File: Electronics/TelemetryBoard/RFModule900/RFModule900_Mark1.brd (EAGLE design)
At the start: 100 x 30 mm, 166 parts, among them T1 DC08-73, T2 DC08-73, U1 TPS2561, U2 TPS2561, U3 LM75B, U4 LTC5505, U5 LTC5505, U6 MCP4728, U7 ADC128D818, U8 MIC5504-3.3YM5, U9 TCA9535, Y1 30 Mhz

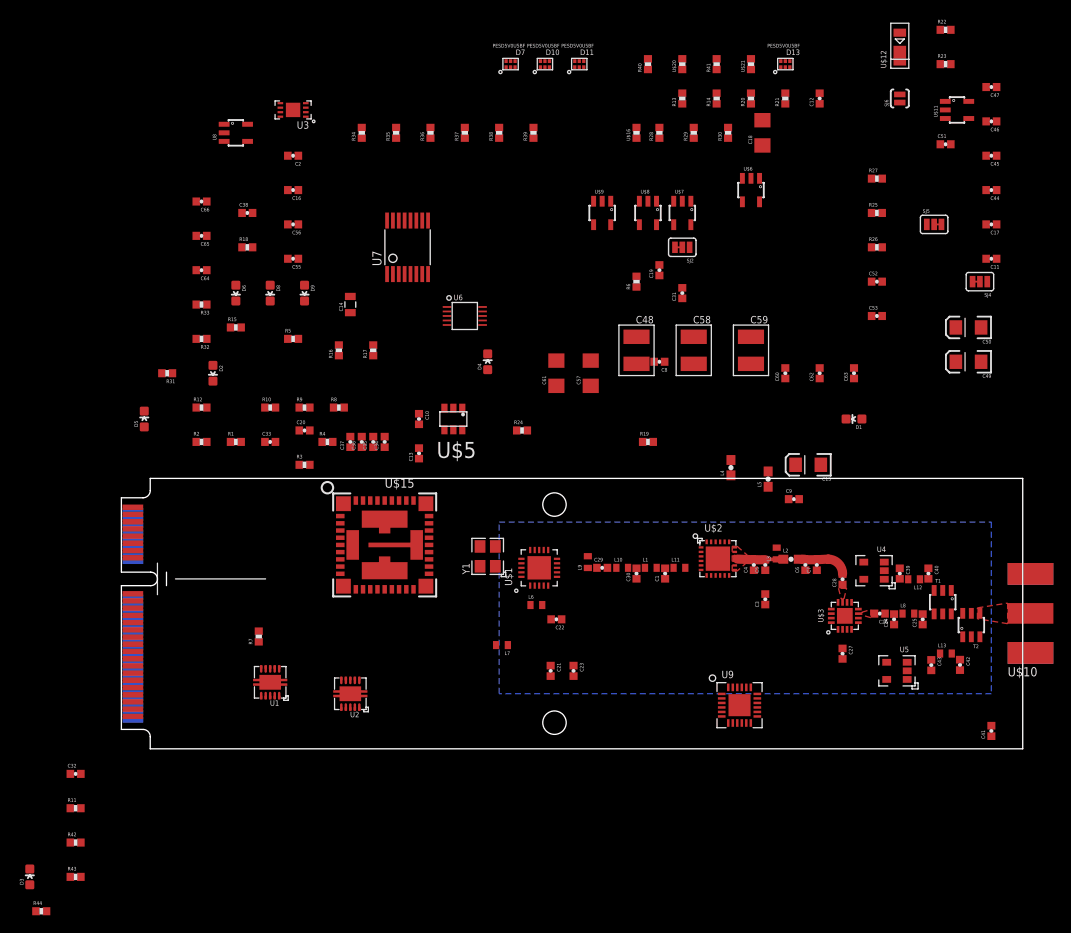
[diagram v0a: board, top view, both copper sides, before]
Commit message: Working on routing board
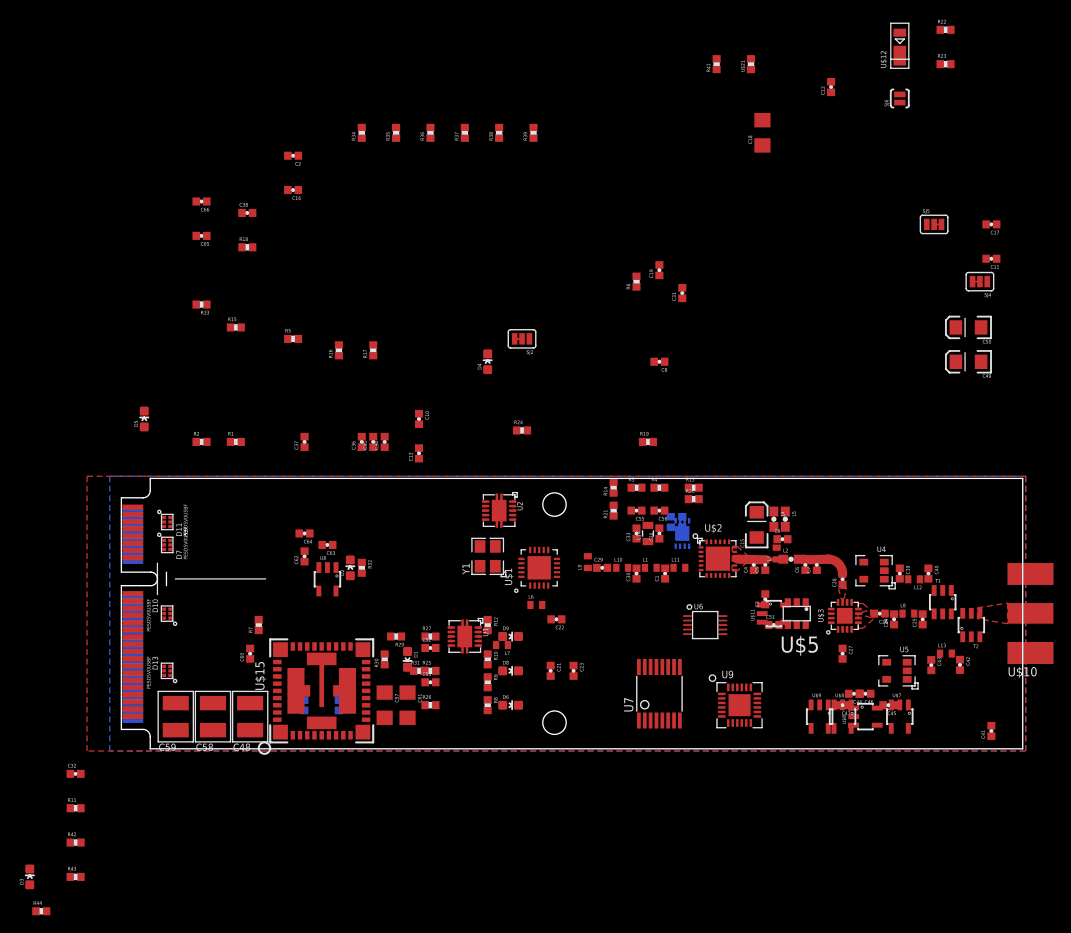
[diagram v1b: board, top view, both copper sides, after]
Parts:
- moved D13 96.1 mm to (5.08, 8.89), turned to 180 degrees
- moved U$20 82.5 mm to (20.3, 5.08), flipped to the bottom
- moved R40 79.0 mm to (24.1, 5.08), flipped to the bottom
- moved C59 75.7 mm to (6.03, 3.81), turned to 270 degrees
- moved D10 74.0 mm to (5.08, 15.2), turned to 180 degrees
- moved R25 70.9 mm to (34.3, 8.89)
- moved R26 70.9 mm to (34.3, 5.08)
- moved R27 70.9 mm to (34.3, 12.7)
- moved C47 70.5 mm to (80.0, 5.08)
- moved R30 69.7 mm to (29.2, 10.2)
- moved D11 68.3 mm to (5.08, 25.4), turned to 0 degrees
- moved C58 67.1 mm to (10.2, 3.81), turned to 270 degrees
- moved C60 67.0 mm to (14.3, 10.8)
- moved D7 65.5 mm to (5.08, 22.9), turned to 0 degrees
- moved C46 65.0 mm to (82.5, 6.35)
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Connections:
- net TR_SWITCH_CTL: now also U$11.2
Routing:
- added copper zone on layer 1, net GND
- added copper zone on layer 15, net GND
- added copper zone on layer 16, net GND
- added copper zone on layer 2, net GND
- removed copper zone on layer 16, net N$3
